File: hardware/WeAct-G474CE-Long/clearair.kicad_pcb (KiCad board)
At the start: 2 copper layers, 90.7 x 71.5 mm, 35 parts, among them J3 SPS30 wire header (1 VDD, 2 S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, J4 BME680 wire header (1 VCC, 2 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, J5 MQ131 wire header (1 VCC, 2 G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, J6 MiCS-4514 wire header (1 VCC,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, M2 80mm fan front, M3 80mm fan rear, Q1 2N7000, Q2 2N7000, Q3 2N2222A, SW1 RESET, SW2 COLD_BOOT, U5 RobotDyn AC dimmer, U6 PCF8563 RTC

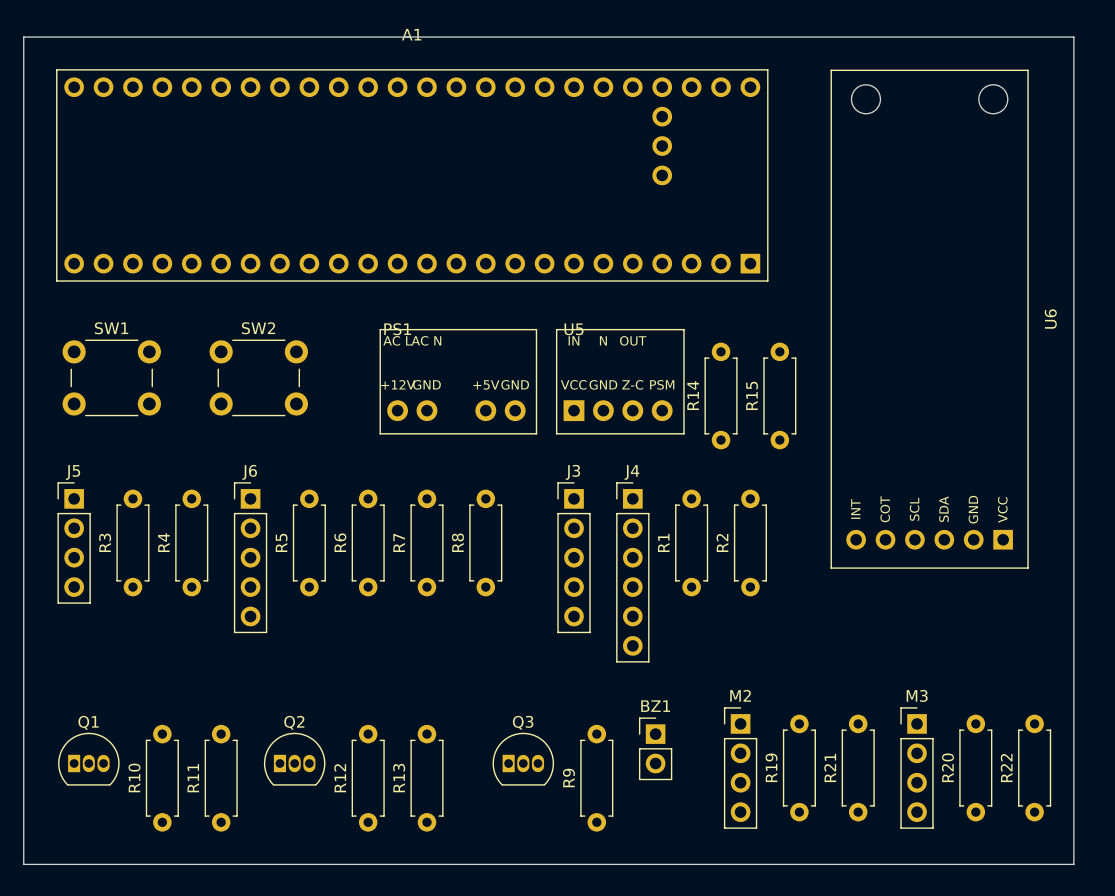
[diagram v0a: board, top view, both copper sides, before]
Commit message: finalize wiring
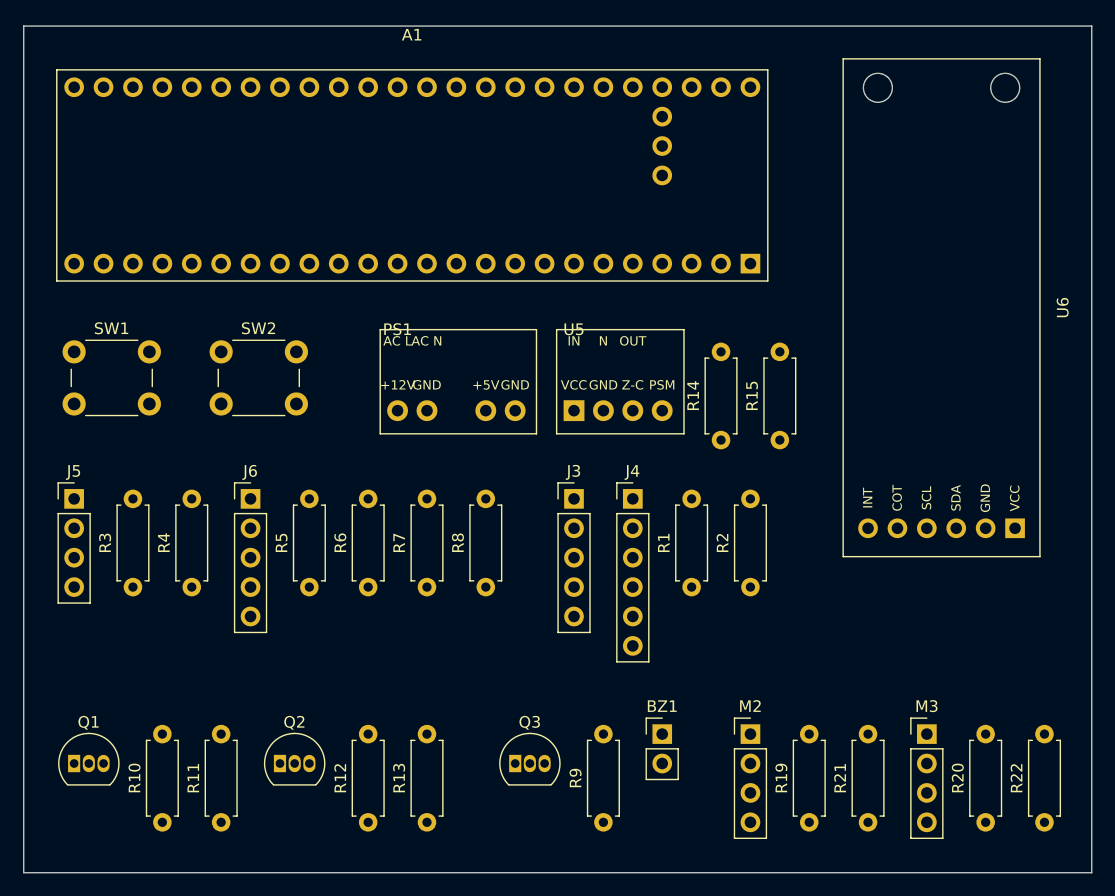
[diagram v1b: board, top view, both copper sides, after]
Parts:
- moved U6 1.43 mm to (176.5, 80.0)
- moved M2 1.22 mm to (160.0, 116.8)
- moved M3 1.22 mm to (175.3, 116.8)
- moved R19 1.22 mm to (165.1, 124.5)
- moved R20 1.22 mm to (180.3, 124.5)
- moved R21 1.22 mm to (170.2, 124.5)
- moved R22 1.22 mm to (185.4, 124.5)
- moved BZ1 0.57 mm to (152.4, 116.8)
- moved Q3 0.57 mm to (139.7, 119.4)
- moved R9 0.57 mm to (147.3, 124.5)
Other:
- board size 90.7 x 71.5 mm -> 92.3 x 73.1 mm
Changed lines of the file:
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@@
 	(footprint "libraries:PCF8563_HW689"
 		(layer "F.Cu")
-		(at 175.5 81 -90)
+		(at 176.53 80.01 -90)
 		(descr "PCF8563 RTC module HW-689, 43 x 17 mm. 6-pin 2.54 mm header on the right short edge, pin 1 (VCC) at the top as seen in the user's photo: VCC GND SDA SCL COT INT. Two mounting holes at the left corners (position approximate from a photo). Pad positions and outline were not measured: check against the board.")
 		(tags "PCF8563 HW-689 RTC module")
@@
 	(footprint "Resistor_THT:R_Axial_DIN0207_L6.3mm_D2.5mm_P7.62mm_Horizontal"
 		(layer "F.Cu")
-		(at 164.25 123.58 90)
+		(at 165.1 124.46 90)
 		(descr "Resistor, Axial_DIN0207 series, Axial, Horizontal, pin pitch=7.62mm, 0.25W = 1/4W, length*diameter=6.3*2.5mm^2, http://cdn-reichelt.de/documents/datenblatt/B400/1_4W%23YAG.pdf")
 		(tags "Resistor Axial_DIN0207 series Axial Horizontal pin pitch 7.62mm 0.25W = 1/4W length 6.3mm diameter 2.5mm")
@@
 	(footprint "Resistor_THT:R_Axial_DIN0207_L6.3mm_D2.5mm_P7.62mm_Horizontal"
 		(layer "F.Cu")
-		(at 169.33 123.58 90)
+		(at 170.18 124.46 90)
 		(descr "Resistor, Axial_DIN0207 series, Axial, Horizontal, pin pitch=7.62mm, 0.25W = 1/4W, length*diameter=6.3*2.5mm^2, http://cdn-reichelt.de/documents/datenblatt/B400/1_4W%23YAG.pdf")
 		(tags "Resistor Axial_DIN0207 series Axial Horizontal pin pitch 7.62mm 0.25W = 1/4W length 6.3mm diameter 2.5mm")
@@
 	(footprint "Resistor_THT:R_Axial_DIN0207_L6.3mm_D2.5mm_P7.62mm_Horizontal"
 		(layer "F.Cu")
-		(at 184.57 123.58 90)
+		(at 185.42 124.46 90)
 		(descr "Resistor, Axial_DIN0207 series, Axial, Horizontal, pin pitch=7.62mm, 0.25W = 1/4W, length*diameter=6.3*2.5mm^2, http://cdn-reichelt.de/documents/datenblatt/B400/1_4W%23YAG.pdf")
 		(tags "Resistor Axial_DIN0207 series Axial Horizontal pin pitch 7.62mm 0.25W = 1/4W length 6.3mm diameter 2.5mm")
@@
 	(footprint "Connector_PinHeader_2.54mm:PinHeader_1x04_P2.54mm_Vertical"
 		(layer "F.Cu")
-		(at 174.41 115.96)
+		(at 175.26 116.84)
 		(descr "Through hole straight pin header, 1x04, 2.54mm pitch, single row")
 		(tags "Through hole pin header THT 1x04 2.54mm single row")
@@
 	(footprint "Connector_PinHeader_2.54mm:PinHeader_1x02_P2.54mm_Vertical"
 		(layer "F.Cu")
-		(at 151.83 116.84)
+		(at 152.4 116.84)
 		(descr "Through hole straight pin header, 1x02, 2.54mm pitch, single row")
 		(tags "Through hole pin header THT 1x02 2.54mm single row")
@@
 	(footprint "Resistor_THT:R_Axial_DIN0207_L6.3mm_D2.5mm_P7.62mm_Horizontal"
 		(layer "F.Cu")
-		(at 179.49 123.58 90)
+		(at 180.34 124.46 90)
 		(descr "Resistor, Axial_DIN0207 series, Axial, Horizontal, pin pitch=7.62mm, 0.25W = 1/4W, length*diameter=6.3*2.5mm^2, http://cdn-reichelt.de/documents/datenblatt/B400/1_4W%23YAG.pdf")
 		(tags "Resistor Axial_DIN0207 series Axial Horizontal pin pitch 7.62mm 0.25W = 1/4W length 6.3mm diameter 2.5mm")
@@
 	(footprint "Package_TO_SOT_THT:TO-92_Inline"
 		(layer "F.Cu")
-		(at 139.13 119.38)
+		(at 139.7 119.38)
 		(descr "TO-92 leads in-line, narrow, oval pads, drill 0.75mm (see NXP sot054_po.pdf)")
 		(tags "to-92 sc-43 sc-43a sot54 PA33 transistor")
@@
 	(footprint "Connector_PinHeader_2.54mm:PinHeader_1x04_P2.54mm_Vertical"
 		(layer "F.Cu")
-		(at 159.17 115.96)
+		(at 160.02 116.84)
 		(descr "Through hole straight pin header, 1x04, 2.54mm pitch, single row")
 		(tags "Through hole pin header THT 1x04 2.54mm single row")
@@
 	(footprint "Resistor_THT:R_Axial_DIN0207_L6.3mm_D2.5mm_P7.62mm_Horizontal"
 		(layer "F.Cu")
-		(at 146.75 124.46 90)
+		(at 147.32 124.46 90)
 		(descr "Resistor, Axial_DIN0207 series, Axial, Horizontal, pin pitch=7.62mm, 0.25W = 1/4W, length*diameter=6.3*2.5mm^2, http://cdn-reichelt.de/documents/datenblatt/B400/1_4W%23YAG.pdf")
 		(tags "Resistor Axial_DIN0207 series Axial Horizontal pin pitch 7.62mm 0.25W = 1/4W length 6.3mm diameter 2.5mm")
@@
 	)
 	(gr_rect
-		(start 97.245 56.625)
-		(end 187.96 128.095)
+		(start 97.245 55.675)
+		(end 189.505 128.815)
 		(stroke
 			(width 0.1)
